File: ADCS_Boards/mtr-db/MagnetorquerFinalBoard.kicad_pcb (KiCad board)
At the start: 4 copper layers, 90.2 x 95.9 mm, 48 parts, among them J1 PC104_Connector, U1 X/Y_Coils, U2 Z_Coil

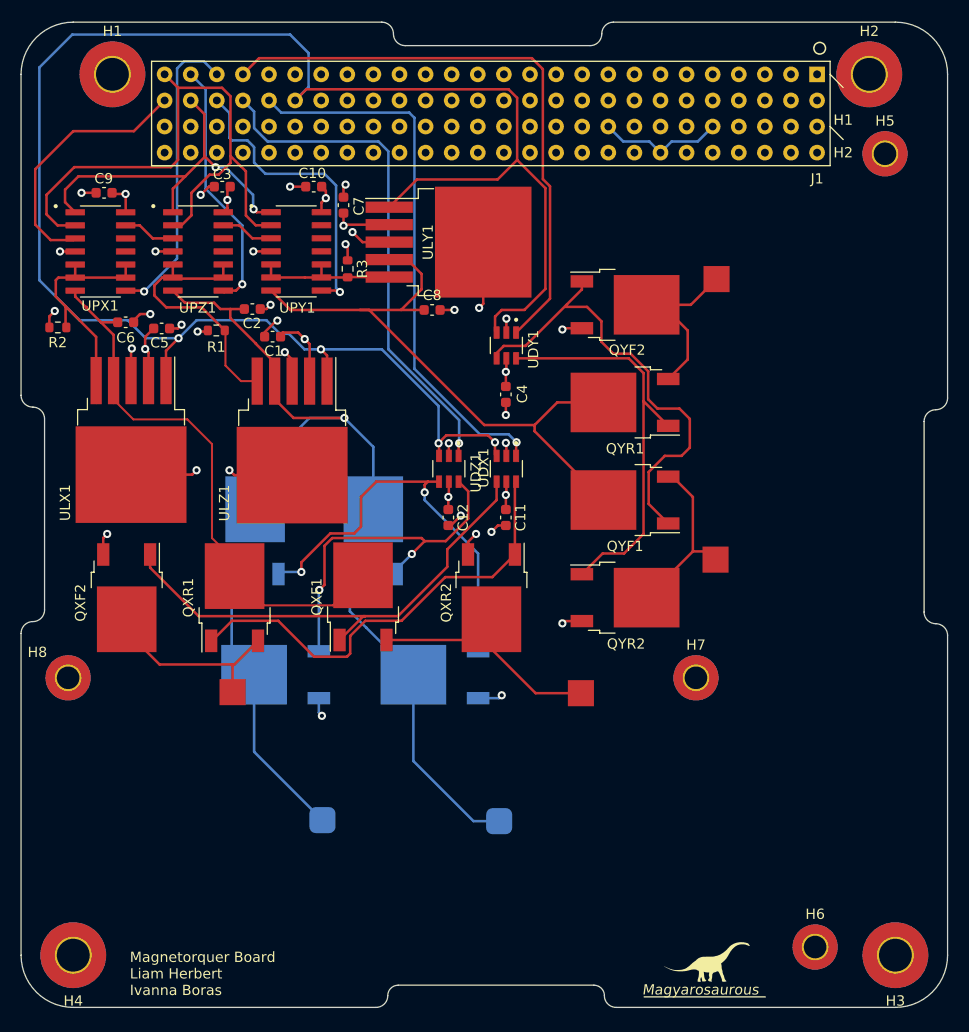
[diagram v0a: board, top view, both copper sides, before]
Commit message: adcs: mtr-db: updated design from Liam
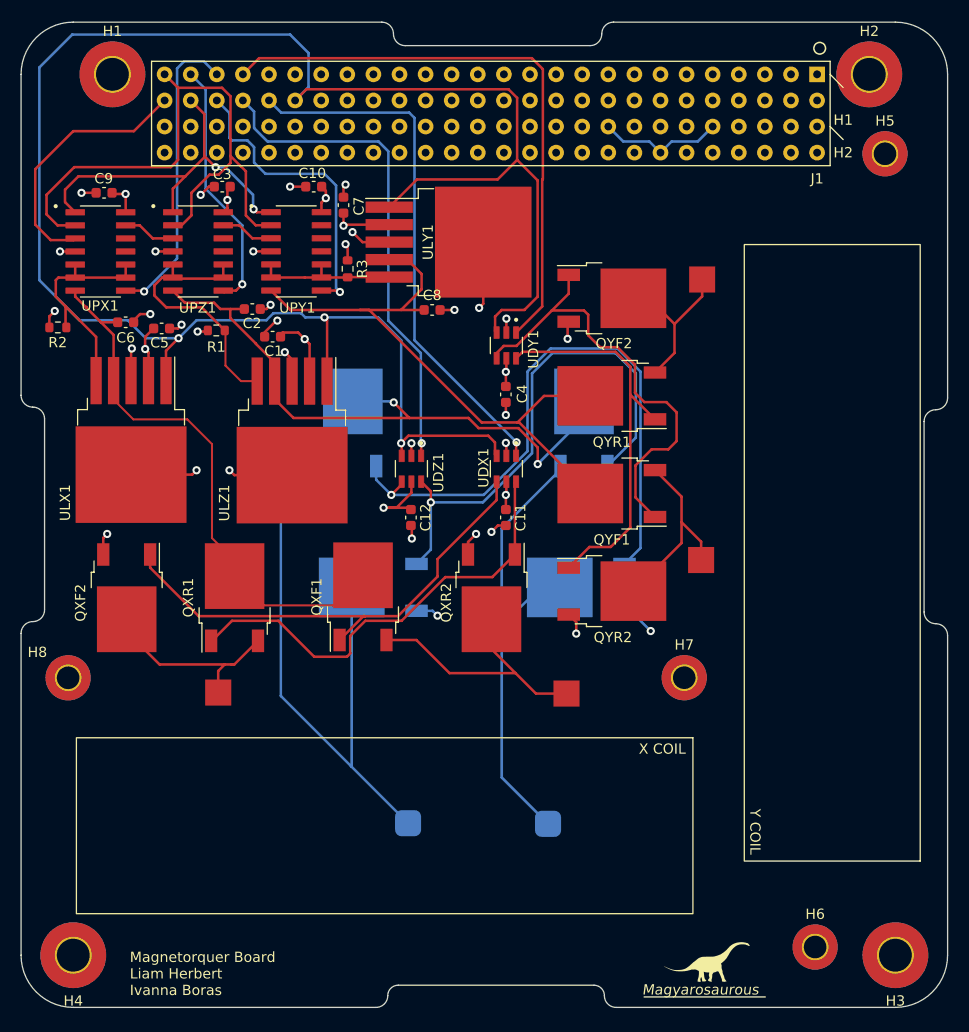
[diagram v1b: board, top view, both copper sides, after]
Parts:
- QXF1, QXF2, QXR1, QXR2, QYF1, QYF2, QYR1, QYR2, QZF1, QZF2, QZR1, QZR2: value IRF540N -> IRLR120N
- moved QZR1 23.0 mm to (164.0, 86.0)
- moved QZF2 16.6 mm to (163.8, 102.0)
- moved QZF1 14.2 mm to (141.5, 86.0)
- moved QZR2 12.7 mm to (143.5, 102.0)
- moved C12 3.64 mm to (147.2, 95.2)
- moved UDZ1 3.64 mm to (147.2, 90.5)
- moved U2 1.47 mm to (189.3, 63.0)
- moved QYF1 1.43 mm to (166.7, 92.9)
- moved QYF2 1.43 mm to (166.7, 73.9)
- moved QYR1 1.43 mm to (166.7, 83.4)
- moved QYR2 1.43 mm to (166.7, 102.4)
- moved U1 1.40 mm to (196.6, 63.6)
- moved H7 1.14 mm to (173.8, 110.8)
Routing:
- net Z_COIL_A: track 27.6 -> 63.6 mm
- net Z_FWD: track 41.8 -> 60.1 mm, vias 2 -> 1
- net Z_REV: track 34.1 -> 50.5 mm, vias 2 -> 1
- net Z_COIL_B: track 31.5 -> 46.2 mm
- net Z_VCOIL: track 52.3 -> 63.6 mm, vias 1 -> 2
- net Enable: track 185.3 -> 191.9 mm, vias 4 -> 3
- net X_COIL_A: track 24.4 -> 28.8 mm
- net 5V: track 37.4 -> 41.4 mm
- net Y_COIL_B: track 18.4 -> 16.0 mm
- net Y_COIL_A: track 17.4 -> 19.7 mm
- net X_S: track 53.5 -> 51.9 mm
- net Z_S: track 49.7 -> 48.2 mm
- net Y_VCOIL: track 63.6 -> 62.3 mm
- net Y_REV: track 39.7 -> 38.6 mm
- net GND: track 88.8 -> 89.7 mm
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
